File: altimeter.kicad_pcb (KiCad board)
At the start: 2 copper layers, 45 x 24 mm, 67 parts, among them J201 Conn_01x10, J202 Conn_ARM_JTAG_SWD_10, J203 Conn_02x03_Counter_Clockwise, J204 USB_B_Micro, J205 Conn_01x04, Q1 BC847BDW1, Q101 DMG2301L, Q102 DMG2301L, Q301 BC847BDW1, Q401 BC847BDW1, Q501 BC847BDW1, U101 STM32F302CCTx, U102 MT25Q, U103 AIS2120SXTR, U104 MIC5219-3.3YM5, U105 LF50_TO252, U107 MS5611-01BA, U2 ICM-20602, U301 SI7232DN, U501 SI7232DN, Y1 Crystal_GND24

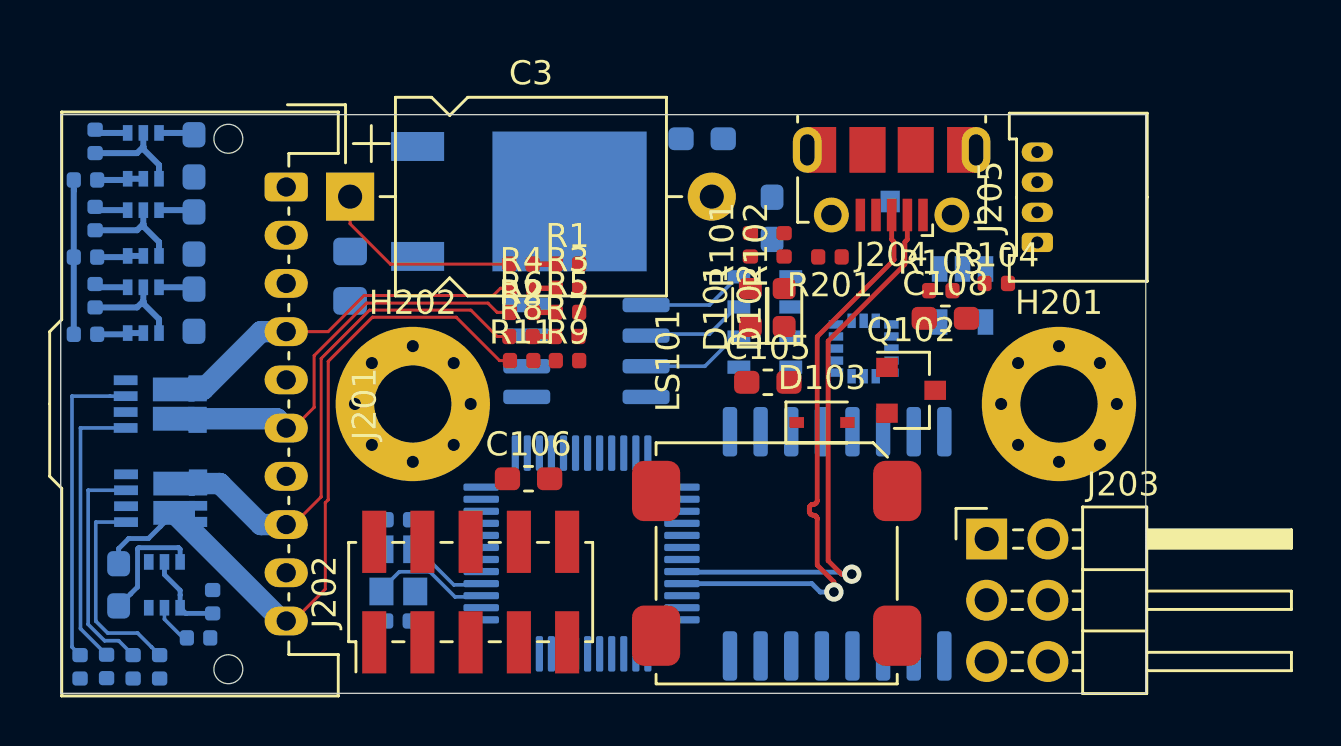
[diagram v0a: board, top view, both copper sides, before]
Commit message: major work on layout. nearly finished
Signed-off-by: Thomas Schmid <tom@binary-kitchen.de>
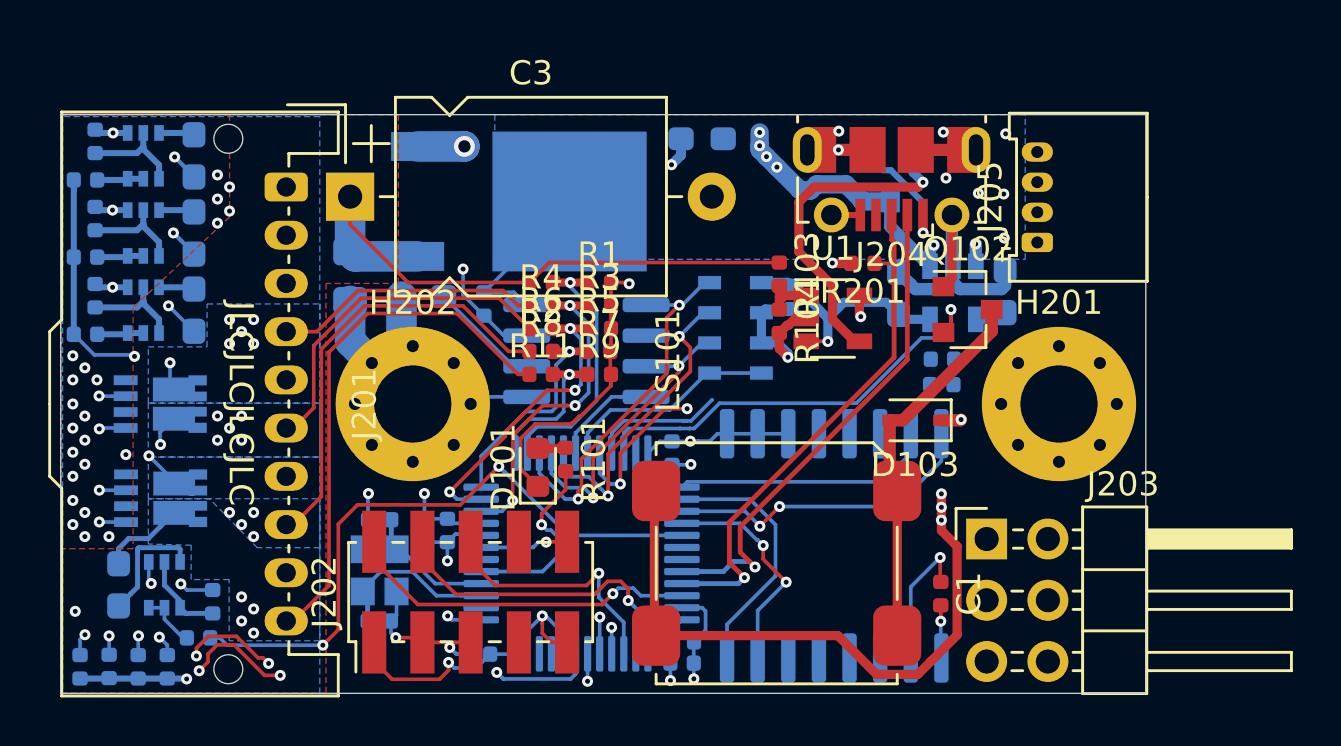
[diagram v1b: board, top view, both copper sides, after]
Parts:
- removed D102: LED, LED_SMD:LED_0603_1608Metric
- removed R102: 680, Resistor_SMD:R_0402_1005Metric
- removed U2: ICM-20602, Package_LGA:LGA-16_3x3mm_P0.5mm_LayoutBorder3x5y
- added C1: 100n, Capacitor_SMD:C_0402_1005Metric, F.Cu at (174.5, 116.9)
- added C109: 100n, Capacitor_SMD:C_0402_1005Metric, B.Cu at (174.5, 108.2)
- added C110: 100n, Capacitor_SMD:C_0402_1005Metric, B.Cu at (174.6, 107.1)
- added C111: C_Small, Capacitor_SMD:C_0402_1005Metric, B.Cu at (163.3, 111.0)
- added C112: C_Small, Capacitor_SMD:C_0402_1005Metric, B.Cu at (153.1, 114.2)
- added C113: C_Small, Capacitor_SMD:C_0402_1005Metric, B.Cu at (155.3, 119.4)
- added C114: C_Small, Capacitor_SMD:C_0402_1005Metric, B.Cu at (154.0, 114.2)
- added C115: C_Small, Capacitor_SMD:C_0402_1005Metric, B.Cu at (163.8, 118.9)
- added C116: C_Small, Capacitor_SMD:C_0402_1005Metric, B.Cu at (163.8, 119.7)
- added C2: 100n, Capacitor_SMD:C_0402_1005Metric, B.Cu at (155.5, 104.9)
- added U1: LMV331, Package_TO_SOT_SMD:SOT-23-5, F.Cu at (170.0, 105.5)
- C105, C108: moved to B.Cu
- C106: footprint Capacitor_SMD:C_0603_1608Metric_Pad1.05x0.95mm_HandSolder -> Capacitor_SMD:C_0402_1005Metric; moved to B.Cu
- U102: value MT25Q -> S25L512S
- moved C103 14.9 mm to (153.0, 104.5), turned to 0 degrees
- moved C106 13.2 mm to (168.3, 104.6), turned to 90 degrees
- moved R101 11.7 mm to (158.9, 111.3), turned to 270 degrees
- moved D101 11.0 mm to (157.8, 111.6)
- moved C105 10.5 mm to (177.2, 104.3), turned to 90 degrees
- moved R104 9.14 mm to (167.8, 105.6), turned to 270 degrees
- moved R103 6.73 mm to (167.8, 103.6), turned to 270 degrees
- moved Q102 4.09 mm to (175.6, 105.1)
- moved D103 3.86 mm to (173.4, 109.7), turned to 180 degrees
- moved C108 2.20 mm to (172.7, 104.4), turned to 90 degrees
- moved R1 1.52 mm to (160.3, 104.0)
- moved R3 1.50 mm to (160.3, 104.9)
- moved R5 1.48 mm to (160.3, 105.9)
- moved R7 1.46 mm to (160.3, 106.8)
- moved R9 1.44 mm to (160.3, 107.8)
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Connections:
- net BARO_CSS renamed IMU_GYRO_CS
- net JTCK renamed SWCLK
- net JTDO renamed SWO
- net JTMS renamed SWDIO
- J202 pad 8: JTDI -> Net-(J202-Pad8)
- U101 pad 18: Net-(U101-Pad18) -> ACC_CS
- U101 pad 19: SUMMER -> BARO_CS
- U101 pad 21: ACC_CS -> IMU_ACC_CS
- U101 pad 22: IMU_CS -> SUMMER
- U101 pad 38: JTDI -> INT1
- U101 pad 6: LED2 -> INT2
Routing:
- net GND: track 4.22 -> 99.7 mm, vias 0 -> 47
- net PYRO_TEST_ENABLE: track 6.40 -> 52.8 mm, vias 0 -> 3
- net +5V: track 0.00 -> 45.6 mm, vias 0 -> 13
- net +3V3: track 0.00 -> 40.0 mm, vias 0 -> 9
- net FIRE_PYRO0: track 13.1 -> 45.2 mm, vias 0 -> 5
- net FIRE_PYRO1: track 11.7 -> 40.4 mm, vias 0 -> 5
- net FIRE_PYRO2: track 9.53 -> 33.2 mm, vias 0 -> 3
- net FIRE_PYRO3: track 8.59 -> 28.4 mm, vias 0 -> 3
- net SUMMER: track 0.00 -> 18.1 mm, vias 0 -> 1
- net PYRO0_HIGH: track 8.42 -> 25.5 mm
- net Net-(D103-Pad2): track 0.00 -> 15.7 mm
- net SWDIO: track 0.00 -> 14.7 mm, vias 0 -> 1
- net Net-(Q101-Pad2): track 0.00 -> 13.8 mm, vias 0 -> 1
- net SPI2_MISO: track 0.00 -> 13.3 mm, vias 0 -> 2
- net PYRO0_SENSE: track 0.93 -> 13.5 mm, vias 0 -> 3
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- added copper zone on In2.Cu, net +3V3
- added copper zone on In2.Cu, net +5V
- added copper zone on B.Cu, net GND
- added copper zone on F.Cu, net GND
- added copper zone on In1.Cu, net GND
- added copper zone on In2.Cu, net GND
- added copper zone on F.Cu, net PYRO0_HIGH
- added copper zone on In1.Cu, net PYRO0_HIGH
- added copper zone on B.Cu, net PYRO0_LOW
- added copper zone on In2.Cu, net PYRO0_LOW
- added copper zone on B.Cu, net PYRO1_LOW
- added copper zone on In2.Cu, net PYRO1_LOW
- added copper zone on B.Cu, net PYRO2_LOW
- added copper zone on In2.Cu, net PYRO2_LOW
- added copper zone on B.Cu, net PYRO3_LOW
- added copper zone on In2.Cu, net PYRO3_LOW
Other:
- copper layers 2 -> 4
- board text added: "JLCJLCJLCJLC"
